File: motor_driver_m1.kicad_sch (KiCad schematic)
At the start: 45 parts, among them J2 Conn_01x01_Pin, J4 Conn_01x01_Pin, J5 Conn_01x01_Pin, J6 Conn_01x01_Pin, Q1 NP80N06D6, Q2 NP80N06D6, Q3 NP80N06D6, Q4 NP80N06D6, Q5 NP80N06D6, Q6 NP80N06D6, U2 STM32C011F6U6TR, U3 STDRIVE101

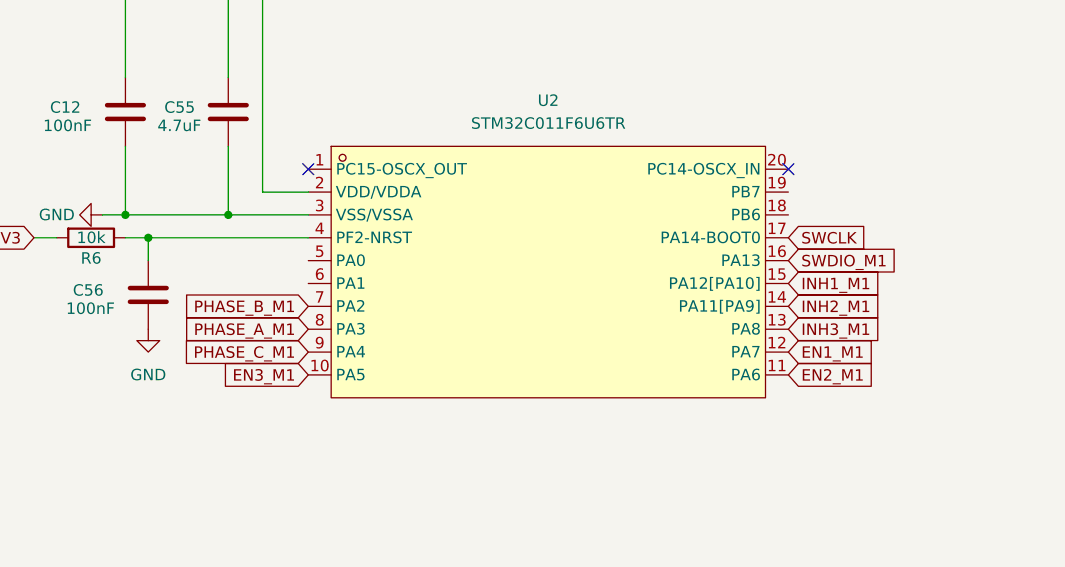
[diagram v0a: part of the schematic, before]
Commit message: ...
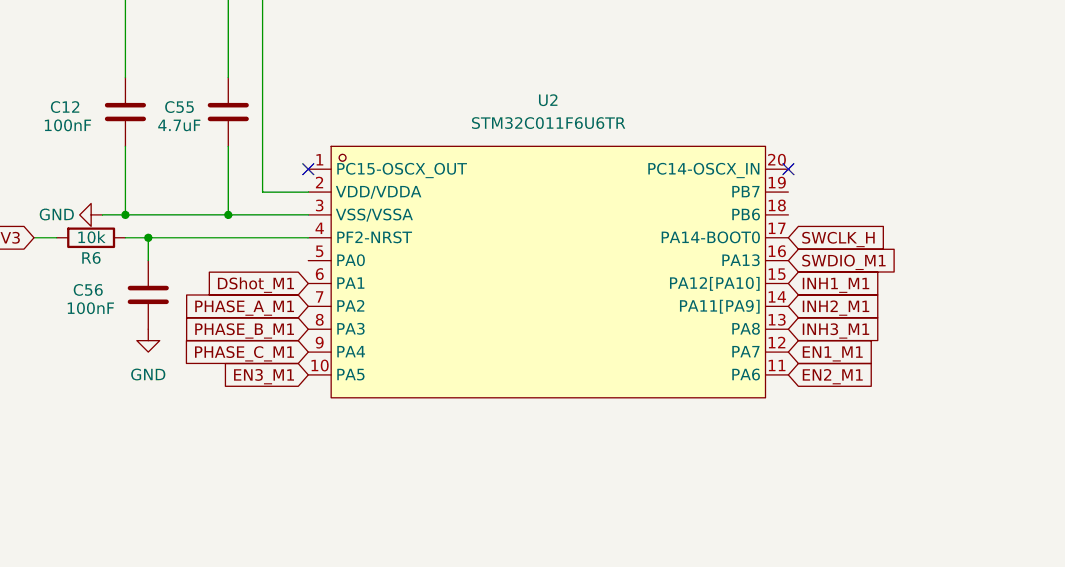
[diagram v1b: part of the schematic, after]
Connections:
- net DShot_M1: now also U2.6 (PA1)
- net PHASE_A_M1: now also U2.7 (PA2); no longer U2.8 (PA3)
- net PHASE_B_M1: now also U2.8 (PA3); no longer U2.7 (PA2)
- net SWCLK renamed SWCLK_H
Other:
- title: (none) -> MOTOR DRIVER M1
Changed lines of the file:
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@@
 	(generator_version "10.0")
 	(paper "A4")
+	(title_block
+		(title "MOTOR DRIVER M1")
+		(rev "1.0")
+	)
 	(text_box "DShot\n"
 		(exclude_from_sim no)
@@
 		)
 	)
+	(global_label "DShot_M1"
+		(shape input)
+		(at 64.77 57.15 180)
+		(fields_autoplaced yes)
+		(effects
+			(font
+				(size 1.27 1.27)
+			)
+			(justify right)
+		)
+		(property "Intersheetrefs" "${INTERSHEET_REFS}"
+			(at 52.6531 57.15 0)
+			(hide yes)
+			(show_name no)
+			(do_not_autoplace no)
+			(effects
+				(font
+					(size 1.27 1.27)
+				)
+				(justify right)
+			)
+		)
+	)
 	(global_label "INH1_M1"
 		(shape input)
@@
 		)
 	)
-	(global_label "PHASE_A_M1"
+	(global_label "PHASE_B_M1"
 		(shape input)
 		(at 64.77 62.23 180)
@@
 		)
 		(property "Intersheetrefs" "${INTERSHEET_REFS}"
-			(at 50.0525 62.23 0)
+			(at 49.8711 62.23 0)
 			(hide yes)
 			(show_name no)
@@
 		)
 	)
-	(global_label "PHASE_B_M1"
+	(global_label "PHASE_A_M1"
 		(shape input)
 		(at 64.77 59.69 180)
@@
 		)
 		(property "Intersheetrefs" "${INTERSHEET_REFS}"
-			(at 49.8711 59.69 0)
+			(at 50.0525 59.69 0)
 			(hide yes)
 			(show_name no)
@@
 		)
 	)
-	(global_label "SWCLK"
+	(global_label "SWCLK_H"
 		(shape input)
 		(at 118.11 52.07 0)
@@
 		)
 		(property "Intersheetrefs" "${INTERSHEET_REFS}"
-			(at 127.3242 52.07 0)
+			(at 129.6223 52.07 0)
 			(hide yes)
 			(show_name no)
